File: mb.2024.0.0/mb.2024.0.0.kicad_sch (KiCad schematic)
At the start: 24 parts, among them J1 DSP_out_12v_GND, J10 DSP+, J11 Screw_Terminal_VMN, J13 Connector_I2C_for_mux, J16 RX_bat, J17 DSP GND, J18 ELEC_M, J19 ELEC_N, J2 DPS5005_input_0_to_50V, J3 Screw_Terminal_AB, J4 Conn_01x08_Female, J5 Conn_01x04_Female, J6 Conn_01x08_Female, J7 Raspberry_Pi_2_3, J8 Connector_I2C_for_MCP23008, J9 TX_bat, U1 MCP23008-xP, U3 24LC02

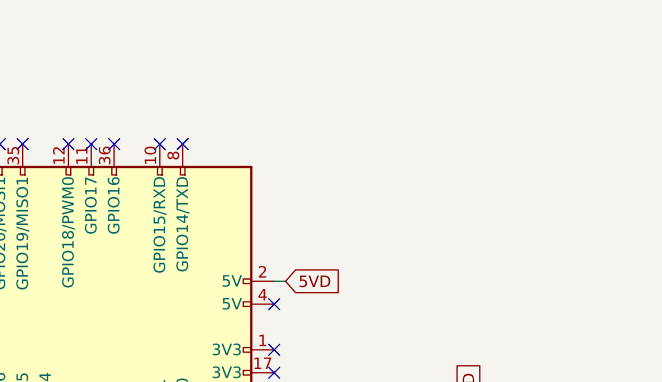
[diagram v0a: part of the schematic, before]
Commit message: update pcb
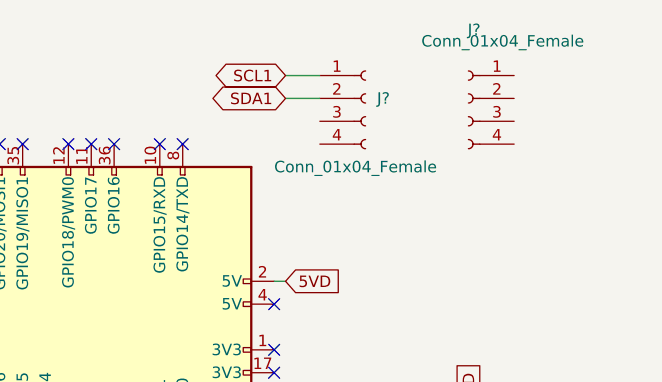
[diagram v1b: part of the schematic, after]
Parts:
- added J? (x2): Conn_01x04_Female, symbol Connector:Conn_01x04_Female
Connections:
- net SCL1: now also J?.1 (Pin_1)
- net SDA1: now also J?.2 (Pin_2)
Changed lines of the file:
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@@
+    (stroke (width 0) (type default) (color 0 0 0 0))
+  )
+  (wire (pts (xy 247.65 20.32) (xy 251.46 20.32))
     (stroke (width 0) (type default) (color 0 0 0 0))
   )
@@
     (stroke (width 0) (type default) (color 0 0 0 0))
   )
+  (wire (pts (xy 247.65 17.78) (xy 251.46 17.78))
+    (stroke (width 0) (type default) (color 0 0 0 0))
+  )
   (wire (pts (xy 142.24 157.48) (xy 138.43 157.48))
     (stroke (width 0) (type default) (color 0 0 0 0))
@@
     )
   )
+  (global_label "SCL1" (shape bidirectional) (at 247.65 17.78 180) (fields_autoplaced)
+    (effects (font (size 1.27 1.27)) (justify right))
+    (property "Intersheet References" "${INTERSHEET_REFS}" (id 0) (at 240.5198 17.7006 0)
+      (effects (font (size 1.27 1.27)) (justify right) hide)
+    )
+  )
   (global_label "GP0" (shape input) (at 64.77 157.48 0) (fields_autoplaced)
     (effects (font (size 1.27 1.27)) (justify left))
@@
     (effects (font (size 1.27 1.27)) (justify right))
     (property "Intersheet References" "${INTERSHEET_REFS}" (id 0) (at 71.4283 24.0506 0)
+      (effects (font (size 1.27 1.27)) (justify right) hide)
+    )
+  )
+  (global_label "SDA1" (shape bidirectional) (at 247.65 20.32 180) (fields_autoplaced)
+    (effects (font (size 1.27 1.27)) (justify right))
+    (property "Intersheet References" "${INTERSHEET_REFS}" (id 0) (at 240.4593 20.2406 0)
       (effects (font (size 1.27 1.27)) (justify right) hide)
     )
@@
     )
     (pin "1")
+  )
+  (symbol (lib_id "Connector:Conn_01x04_Female") (at 267.97 20.32 0) (mirror y) (unit 1)
+    (in_bom yes) (on_board yes)
+    (property "Reference" "J?" (id 0) (at 268.605 12.7 0))
+    (property "Value" "Conn_01x04_Female" (id 1) (at 271.78 13.97 0))
+    (property "Footprint" "" (id 2) (at 267.97 20.32 0)
+      (effects (font (size 1.27 1.27)) hide)
+    )
+    (property "Datasheet" "~" (id 3) (at 267.97 20.32 0)
+      (effects (font (size 1.27 1.27)) hide)
+    )
+    (pin "1")
+    (pin "2")
+    (pin "3")
+    (pin "4")
   )
   (symbol (lib_id "Device:R") (at 137.16 116.84 0) (unit 1)
@@
     (pin "9")
   )
+  (symbol (lib_id "Connector:Conn_01x04_Female") (at 256.54 20.32 0) (unit 1)
+    (in_bom yes) (on_board yes)
+    (property "Reference" "J?" (id 0) (at 257.81 20.3199 0)
+      (effects (font (size 1.27 1.27)) (justify left))
+    )
+    (property "Value" "Conn_01x04_Female" (id 1) (at 246.38 27.94 0)
+      (effects (font (size 1.27 1.27)) (justify left))
+    )
+    (property "Footprint" "" (id 2) (at 256.54 20.32 0)
+      (effects (font (size 1.27 1.27)) hide)
+    )
+    (property "Datasheet" "~" (id 3) (at 256.54 20.32 0)
+      (effects (font (size 1.27 1.27)) hide)
+    )
+    (pin "1")
+    (pin "2")
+    (pin "3")
+    (pin "4")
+  )
   (symbol (lib_id "power:GNDD") (at 255.27 81.28 0) (unit 1)
     (in_bom yes) (on_board yes) (fields_autoplaced)
@@
       (reference "J21") (unit 1) (value "shunt -") (footprint "Connector_PinHeader_2.54mm:PinHeader_1x01_P2.54mm_Vertical")
     )
+    (path "/15a23eee-5975-4755-b1b0-cd09ad193c00"
+      (reference "J?") (unit 1) (value "Conn_01x04_Female") (footprint "")
+    )
+    (path "/99ab4477-5bb9-4eb2-ada0-903b9f73815a"
+      (reference "J?") (unit 1) (value "Conn_01x04_Female") (footprint "")
+    )
     (path "/433fb79c-38b7-4d80-8278-5eb2a5e83393/3be27309-3160-4185-86f9-1c67d16e946d"
